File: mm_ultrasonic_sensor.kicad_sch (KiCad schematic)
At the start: 0 parts

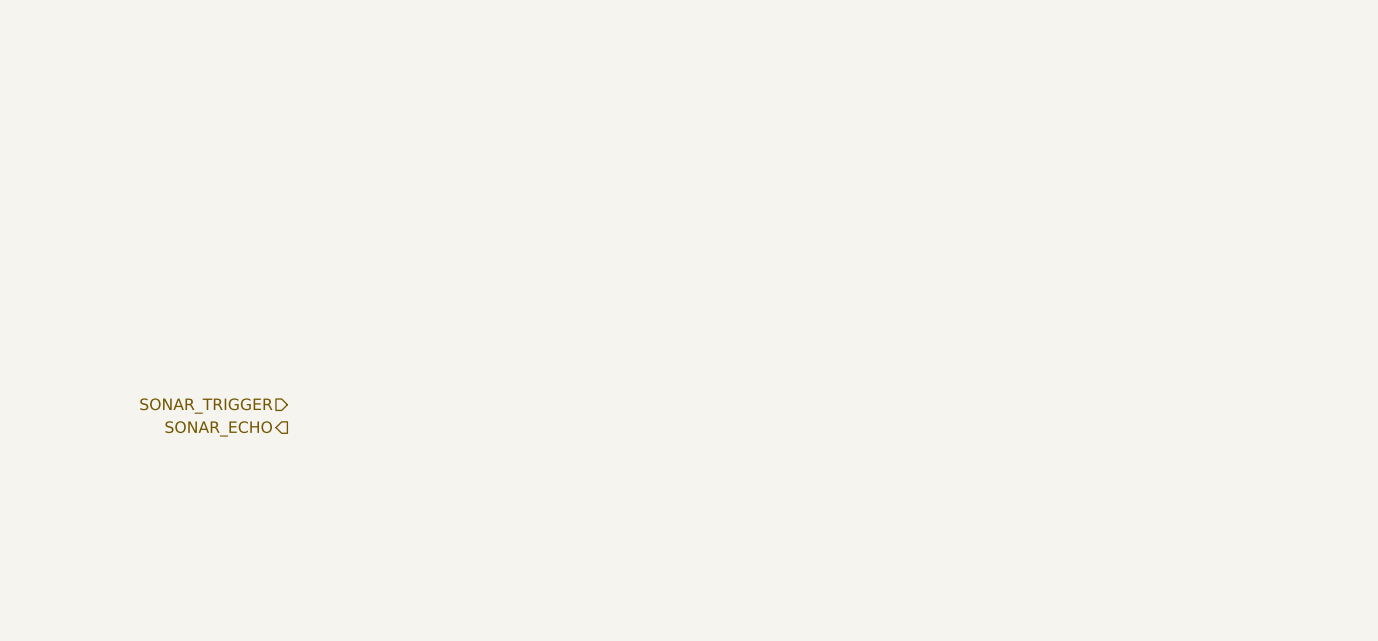
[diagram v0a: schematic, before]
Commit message: tp2
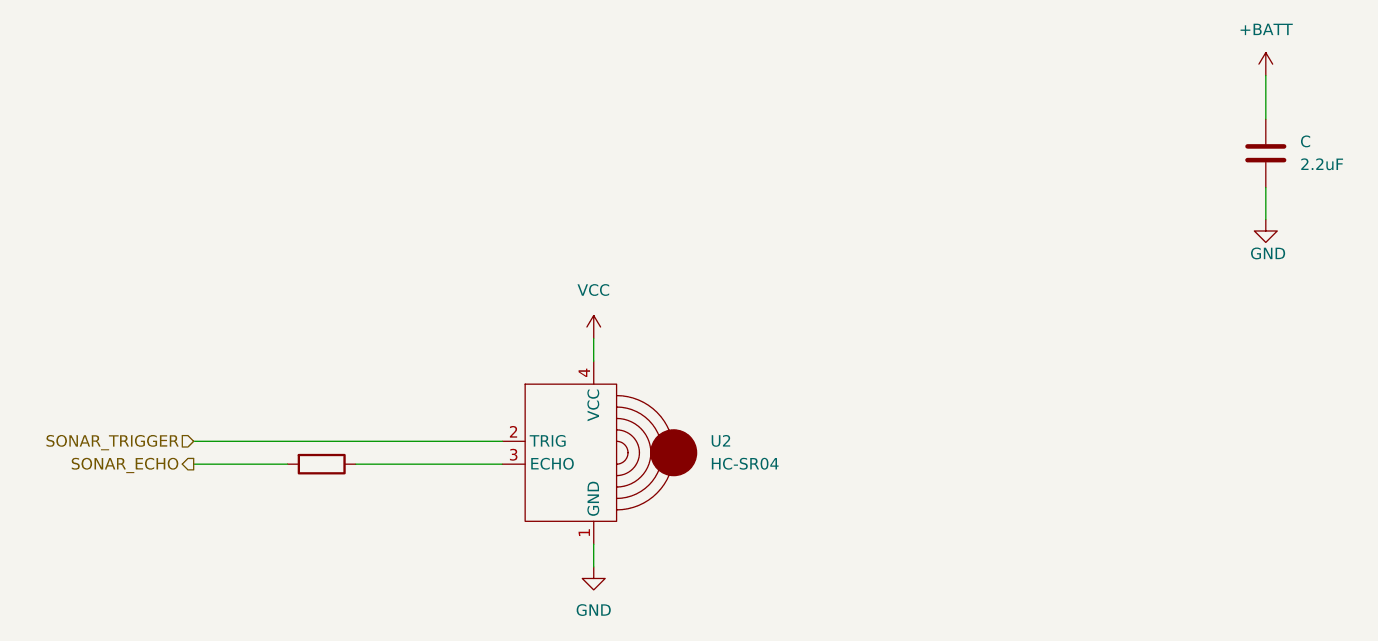
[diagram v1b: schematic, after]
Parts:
- added C: 2.2uF, symbol Device:C
- added R12: 100, symbol Device:R
- added U2: HC-SR04, minimouse:HC-SR04, symbol minimouse:HC-SR04
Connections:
- net SONAR_ECHO: now also R12.2
- net SONAR_TRIGGER: now also U2.2 (TRIG)
- new net: R12.1, U2.3 (ECHO)
- new net +BATT: C.1
- new net GND: C.2, U2.1 (GND)
- new net VCC: U2.4 (VCC)
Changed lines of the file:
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@@
 (kicad_sch (version 20230121) (generator eeschema)
   (paper "A4")
-  (hierarchical_label "SONAR_TRIGGER" (shape input) (at 109.22 88.9 180) (fields_autoplaced)
+  (wire (pts (xy 98.806 92.964) (xy 133.096 92.964))
+    (stroke (width 0) (type default))
+  )
+  (wire (pts (xy 143.256 104.394) (xy 143.256 106.934))
+    (stroke (width 0) (type default))
+  )
+  (wire (pts (xy 217.932 52.324) (xy 217.932 57.15))
+    (stroke (width 0) (type default))
+  )
+  (wire (pts (xy 143.256 81.534) (xy 143.256 84.074))
+    (stroke (width 0) (type default))
+  )
+  (wire (pts (xy 98.806 95.504) (xy 109.22 95.504))
+    (stroke (width 0) (type default))
+  )
+  (wire (pts (xy 217.932 64.77) (xy 217.932 68.326))
+    (stroke (width 0) (type default))
+  )
+  (wire (pts (xy 116.84 95.504) (xy 133.096 95.504))
+    (stroke (width 0) (type default))
+  )
+  (hierarchical_label "SONAR_TRIGGER" (shape input) (at 98.806 92.964 180) (fields_autoplaced)
     (effects (font (size 1.27 1.27)) (justify right))
   )
-  (hierarchical_label "SONAR_ECHO" (shape output) (at 109.22 91.44 180) (fields_autoplaced)
+  (hierarchical_label "SONAR_ECHO" (shape output) (at 98.806 95.504 180) (fields_autoplaced)
     (effects (font (size 1.27 1.27)) (justify right))
   )
+  (symbol (lib_id "power:VCC") (at 143.256 81.534 0) (unit 1)
+    (in_bom yes) (on_board yes) (dnp no) (fields_autoplaced)
+    (property "Reference" "#PWR025" (at 143.256 85.344 0)
+      (effects (font (size 1.27 1.27)) hide)
+    )
+    (property "Value" "VCC" (at 143.256 76.2 0)
+      (effects (font (size 1.27 1.27)))
+    )
+    (property "Footprint" "" (at 143.256 81.534 0)
+      (effects (font (size 1.27 1.27)) hide)
+    )
+    (property "Datasheet" "" (at 143.256 81.534 0)
+      (effects (font (size 1.27 1.27)) hide)
+    )
+    (pin "1")
+    (instances
+      (project "minimouse"
+        (path "/d8fa4cba-2469-4231-847f-065b6b829f44/224298a9-7d6e-4a70-a0a5-f2614895ec28"
+          (reference "#PWR025") (unit 1)
+        )
+      )
+    )
+  )
+  (symbol (lib_id "Device:R") (at 113.03 95.504 270) (unit 1)
+    (in_bom yes) (on_board yes) (dnp no) (fields_autoplaced)
+    (property "Reference" "R12" (at 113.03 90.17 90)
+      (effects (font (size 1.27 1.27)) hide)
+    )
+    (property "Value" "100" (at 113.03 92.71 90)
+      (effects (font (size 1.27 1.27)) hide)
+    )
+    (property "Footprint" "" (at 113.03 93.726 90)
+      (effects (font (size 1.27 1.27)) hide)
+    )
+    (property "Datasheet" "~" (at 113.03 95.504 0)
+      (effects (font (size 1.27 1.27)) hide)
+    )
+    (pin "1")
+    (pin "2")
+    (instances
+      (project "minimouse"
+        (path "/d8fa4cba-2469-4231-847f-065b6b829f44/224298a9-7d6e-4a70-a0a5-f2614895ec28"
+          (reference "R12") (unit 1)
+        )
+      )
+    )
+  )
+  (symbol (lib_id "minimouse:HC-SR04") (at 143.256 94.234 0) (unit 1)
+    (in_bom yes) (on_board yes) (dnp no) (fields_autoplaced)
+    (property "Reference" "U2" (at 156.21 92.964 0)
+      (effects (font (size 1.27 1.27)) (justify left))
+    )
+    (property "Value" "HC-SR04" (at 156.21 95.504 0)
+      (effects (font (size 1.27 1.27)) (justify left))
+    )
+    (property "Footprint" "minimouse:HC-SR04" (at 143.256 94.234 0)
+      (effects (font (size 1.27 1.27)) hide)
+    )
+    (property "Datasheet" "" (at 143.256 94.234 0)
+      (effects (font (size 1.27 1.27)) hide)
+    )
+    (pin "1")
+    (pin "4")
+    (pin "2")
+    (pin "3")
+    (instances
+      (project "minimouse"
+        (path "/d8fa4cba-2469-4231-847f-065b6b829f44/224298a9-7d6e-4a70-a0a5-f2614895ec28"
+          (reference "U2") (unit 1)
+        )
+      )
+    )
+  )
+  (symbol (lib_id "power:GND") (at 143.256 106.934 0) (unit 1)
+    (in_bom yes) (on_board yes) (dnp no) (fields_autoplaced)
+    (property "Reference" "#PWR024" (at 143.256 113.284 0)
+      (effects (font (size 1.27 1.27)) hide)
+    )
+    (property "Value" "GND" (at 143.256 111.76 0)
+      (effects (font (size 1.27 1.27)))
+    )
+    (property "Footprint" "" (at 143.256 106.934 0)
+      (effects (font (size 1.27 1.27)) hide)
+    )
+    (property "Datasheet" "" (at 143.256 106.934 0)
+      (effects (font (size 1.27 1.27)) hide)
+    )
+    (pin "1")
+    (instances
+      (project "minimouse"
+        (path "/d8fa4cba-2469-4231-847f-065b6b829f44/224298a9-7d6e-4a70-a0a5-f2614895ec28"
+          (reference "#PWR024") (unit 1)
+        )
+      )
+    )
+  )
+  (symbol (lib_id "power:+BATT") (at 217.932 52.324 0) (unit 1)
+    (in_bom yes) (on_board yes) (dnp no) (fields_autoplaced)
+    (property "Reference" "#PWR014" (at 217.932 56.134 0)
+      (effects (font (size 1.27 1.27)) hide)
+    )
+    (property "Value" "+BATT" (at 217.932 47.244 0)
+      (effects (font (size 1.27 1.27)))
+    )
+    (property "Footprint" "" (at 217.932 52.324 0)
+      (effects (font (size 1.27 1.27)) hide)
+    )
+    (property "Datasheet" "" (at 217.932 52.324 0)
+      (effects (font (size 1.27 1.27)) hide)
+    )
+    (pin "1")
+    (instances
+      (project "minimouse"
+        (path "/d8fa4cba-2469-4231-847f-065b6b829f44/d17bb1c7-f68a-465e-9a17-5858ef86fc30"
+          (reference "#PWR014") (unit 1)
+        )
+        (path "/d8fa4cba-2469-4231-847f-065b6b829f44/224298a9-7d6e-4a70-a0a5-f2614895ec28"
+          (reference "#PWR033") (unit 1)
+        )
+      )
+    )
+  )
+  (symbol (lib_id "Device:C") (at 217.932 60.96 0) (unit 1)
+    (in_bom yes) (on_board yes) (dnp no) (fields_autoplaced)
+    (property "Reference" "C" (at 221.742 59.69 0)
+      (effects (font (size 1.27 1.27)) (justify left))
+    )
+    (property "Value" "2.2uF" (at 221.742 62.23 0)
+      (effects (font (size 1.27 1.27)) (justify left))
+    )
+    (property "Footprint" "" (at 218.8972 64.77 0)
+      (effects (font (size 1.27 1.27)) hide)
+    )
+    (property "Datasheet" "~" (at 217.932 60.96 0)
+      (effects (font (size 1.27 1.27)) hide)
+    )
+    (pin "2")
+    (pin "1")
+    (instances
+      (project "minimouse"
+        (path "/d8fa4cba-2469-4231-847f-065b6b829f44/d17bb1c7-f68a-465e-9a17-5858ef86fc30"
+          (reference "C") (unit 1)
+        )
+        (path "/d8fa4cba-2469-4231-847f-065b6b829f44/224298a9-7d6e-4a70-a0a5-f2614895ec28"
+          (reference "C9") (unit 1)
+        )
+      )
+    )
+  )
+  (symbol (lib_id "power:GND") (at 217.932 68.326 0) (unit 1)
+    (in_bom yes) (on_board yes) (dnp no)
+    (property "Reference" "#PWR028" (at 217.932 74.676 0)
+      (effects (font (size 1.27 1.27)) hide)
+    )
+    (property "Value" "GND" (at 218.186 72.136 0)
+      (effects (font (size 1.27 1.27)))
+    )
+    (property "Footprint" "" (at 217.932 68.326 0)
+      (effects (font (size 1.27 1.27)) hide)
+    )
+    (property "Datasheet" "" (at 217.932 68.326 0)
+      (effects (font (size 1.27 1.27)) hide)
+    )
+    (pin "1")
+    (instances
+      (project "minimouse"
+        (path "/d8fa4cba-2469-4231-847f-065b6b829f44/d17bb1c7-f68a-465e-9a17-5858ef86fc30"
+          (reference "#PWR028") (unit 1)
+        )
+        (path "/d8fa4cba-2469-4231-847f-065b6b829f44/224298a9-7d6e-4a70-a0a5-f2614895ec28"
+          (reference "#PWR034") (unit 1)
+        )
+      )
+    )
+  )
 )

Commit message: TP3
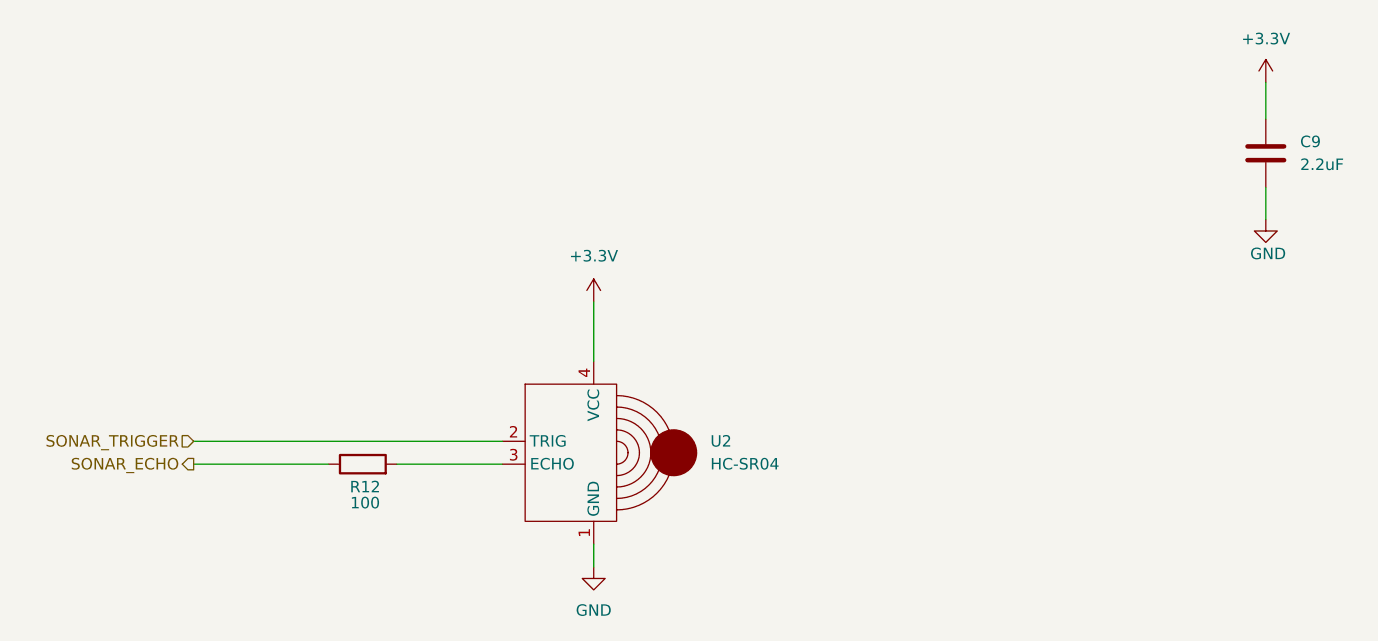
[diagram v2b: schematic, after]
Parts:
- C9: renamed from C; footprint (none) -> Capacitor_SMD:C_0603_1608Metric
- R12: footprint (none) -> Resistor_SMD:R_0603_1608Metric
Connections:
- net VCC is gone; now on net +3.3V: U2.4 (VCC)
- net SONAR_ECHO: now also R12.1; no longer R12.2
- net at U2.3 (ECHO): now also R12.2; no longer R12.1
- net +BATT renamed +3.3V
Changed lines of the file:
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@@
+    (stroke (width 0) (type default))
+  )
+  (wire (pts (xy 121.412 95.504) (xy 133.096 95.504))
     (stroke (width 0) (type default))
   )
@@
     (stroke (width 0) (type default))
   )
-  (wire (pts (xy 217.932 52.324) (xy 217.932 57.15))
+  (wire (pts (xy 143.256 77.47) (xy 143.256 84.074))
     (stroke (width 0) (type default))
   )
-  (wire (pts (xy 143.256 81.534) (xy 143.256 84.074))
+  (wire (pts (xy 98.806 95.504) (xy 113.792 95.504))
     (stroke (width 0) (type default))
   )
-  (wire (pts (xy 98.806 95.504) (xy 109.22 95.504))
+  (wire (pts (xy 217.932 53.086) (xy 217.932 57.15))
     (stroke (width 0) (type default))
   )
   (wire (pts (xy 217.932 64.77) (xy 217.932 68.326))
-    (stroke (width 0) (type default))
-  )
-  (wire (pts (xy 116.84 95.504) (xy 133.096 95.504))
     (stroke (width 0) (type default))
   )
@@
     (effects (font (size 1.27 1.27)) (justify right))
   )
-  (symbol (lib_id "power:VCC") (at 143.256 81.534 0) (unit 1)
-    (in_bom yes) (on_board yes) (dnp no) (fields_autoplaced)
-    (property "Reference" "#PWR025" (at 143.256 85.344 0)
+  (symbol (lib_id "Device:R") (at 117.602 95.504 90) (unit 1)
+    (in_bom yes) (on_board yes) (dnp no)
+    (property "Reference" "R12" (at 117.856 98.044 90)
+      (effects (font (size 1.27 1.27)))
+    )
+    (property "Value" "100" (at 117.856 99.822 90)
+      (effects (font (size 1.27 1.27)))
+    )
+    (property "Footprint" "Resistor_SMD:R_0603_1608Metric" (at 117.602 97.282 90)
       (effects (font (size 1.27 1.27)) hide)
     )
-    (property "Value" "VCC" (at 143.256 76.2 0)
-      (effects (font (size 1.27 1.27)))
-    )
-    (property "Footprint" "" (at 143.256 81.534 0)
+    (property "Datasheet" "~" (at 117.602 95.504 0)
       (effects (font (size 1.27 1.27)) hide)
     )
-    (property "Datasheet" "" (at 143.256 81.534 0)
-      (effects (font (size 1.27 1.27)) hide)
-    )
+    (pin "2")
     (pin "1")
-    (instances
-      (project "minimouse"
-        (path "/d8fa4cba-2469-4231-847f-065b6b829f44/224298a9-7d6e-4a70-a0a5-f2614895ec28"
-          (reference "#PWR025") (unit 1)
-        )
-      )
-    )
-  )
-  (symbol (lib_id "Device:R") (at 113.03 95.504 270) (unit 1)
-    (in_bom yes) (on_board yes) (dnp no) (fields_autoplaced)
-    (property "Reference" "R12" (at 113.03 90.17 90)
-      (effects (font (size 1.27 1.27)) hide)
-    )
-    (property "Value" "100" (at 113.03 92.71 90)
-      (effects (font (size 1.27 1.27)) hide)
-    )
-    (property "Footprint" "" (at 113.03 93.726 90)
-      (effects (font (size 1.27 1.27)) hide)
-    )
-    (property "Datasheet" "~" (at 113.03 95.504 0)
-      (effects (font (size 1.27 1.27)) hide)
-    )
-    (pin "1")
-    (pin "2")
     (instances
       (project "minimouse"
@@
     )
   )
-  (symbol (lib_id "power:+BATT") (at 217.932 52.324 0) (unit 1)
-    (in_bom yes) (on_board yes) (dnp no) (fields_autoplaced)
-    (property "Reference" "#PWR014" (at 217.932 56.134 0)
-      (effects (font (size 1.27 1.27)) hide)
-    )
-    (property "Value" "+BATT" (at 217.932 47.244 0)
-      (effects (font (size 1.27 1.27)))
-    )
-    (property "Footprint" "" (at 217.932 52.324 0)
-      (effects (font (size 1.27 1.27)) hide)
-    )
-    (property "Datasheet" "" (at 217.932 52.324 0)
-      (effects (font (size 1.27 1.27)) hide)
-    )
-    (pin "1")
-    (instances
-      (project "minimouse"
-        (path "/d8fa4cba-2469-4231-847f-065b6b829f44/d17bb1c7-f68a-465e-9a17-5858ef86fc30"
-          (reference "#PWR014") (unit 1)
-        )
-        (path "/d8fa4cba-2469-4231-847f-065b6b829f44/224298a9-7d6e-4a70-a0a5-f2614895ec28"
-          (reference "#PWR033") (unit 1)
-        )
-      )
-    )
-  )
   (symbol (lib_id "Device:C") (at 217.932 60.96 0) (unit 1)
     (in_bom yes) (on_board yes) (dnp no) (fields_autoplaced)
-    (property "Reference" "C" (at 221.742 59.69 0)
+    (property "Reference" "C9" (at 221.742 59.69 0)
       (effects (font (size 1.27 1.27)) (justify left))
     )
@@
       (effects (font (size 1.27 1.27)) (justify left))
     )
-    (property "Footprint" "" (at 218.8972 64.77 0)
+    (property "Footprint" "Capacitor_SMD:C_0603_1608Metric" (at 218.8972 64.77 0)
       (effects (font (size 1.27 1.27)) hide)
     )
@@
     (instances
       (project "minimouse"
-        (path "/d8fa4cba-2469-4231-847f-065b6b829f44/d17bb1c7-f68a-465e-9a17-5858ef86fc30"
-          (reference "C") (unit 1)
-        )
         (path "/d8fa4cba-2469-4231-847f-065b6b829f44/224298a9-7d6e-4a70-a0a5-f2614895ec28"
           (reference "C9") (unit 1)
@@
   (symbol (lib_id "power:GND") (at 217.932 68.326 0) (unit 1)
     (in_bom yes) (on_board yes) (dnp no)
-    (property "Reference" "#PWR028" (at 217.932 74.676 0)
+    (property "Reference" "#PWR034" (at 217.932 74.676 0)
       (effects (font (size 1.27 1.27)) hide)
     )
@@
     (instances
       (project "minimouse"
-        (path "/d8fa4cba-2469-4231-847f-065b6b829f44/d17bb1c7-f68a-465e-9a17-5858ef86fc30"
-          (reference "#PWR028") (unit 1)
-        )
         (path "/d8fa4cba-2469-4231-847f-065b6b829f44/224298a9-7d6e-4a70-a0a5-f2614895ec28"
           (reference "#PWR034") (unit 1)
         )
       )
+    )
+  )
+  (symbol (lib_id "power:+3.3V") (at 143.256 77.47 0) (unit 1)
+    (in_bom yes) (on_board yes) (dnp no) (fields_autoplaced)
+    (property "Reference" "#PWR025" (at 143.256 81.28 0)
+      (effects (font (size 1.27 1.27)) hide)
+    )
+    (property "Value" "+3.3V" (at 143.256 72.39 0)
+      (effects (font (size 1.27 1.27)))
+    )
+    (property "Footprint" "" (at 143.256 77.47 0)
+      (effects (font (size 1.27 1.27)) hide)
+    )
+    (property "Datasheet" "" (at 143.256 77.47 0)
+      (effects (font (size 1.27 1.27)) hide)
+    )
+    (pin "1")
+    (instances
+      (project "minimouse"
+        (path "/d8fa4cba-2469-4231-847f-065b6b829f44/224298a9-7d6e-4a70-a0a5-f2614895ec28"
+          (reference "#PWR025") (unit 1)
+        )
+      )
+    )
+  )
+  (symbol (lib_id "power:+3.3V") (at 217.932 53.086 0) (unit 1)
+    (in_bom yes) (on_board yes) (dnp no) (fields_autoplaced)
+    (property "Reference" "#PWR011" (at 217.932 56.896 0)
+      (effects (font (size 1.27 1.27)) hide)
+    )
+    (property "Value" "+3.3V" (at 217.932 48.26 0)
+      (effects (font (size 1.27 1.27)))
+    )
+    (property "Footprint" "" (at 217.932 53.086 0)
+      (effects (font (size 1.27 1.27)) hide)
+    )
+    (property "Datasheet" "" (at 217.932 53.086 0)
+      (effects (font (size 1.27 1.27)) hide)
+    )
+    (pin "1")
+    (instances
+      (project "minimouse"
+        (path "/d8fa4cba-2469-4231-847f-065b6b829f44/224298a9-7d6e-4a70-a0a5-f2614895ec28"
+          (reference "#PWR011") (unit 1)
+        )
+      )
